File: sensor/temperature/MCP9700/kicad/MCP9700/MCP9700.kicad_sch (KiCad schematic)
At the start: 13 parts, among them U1 MCP9700x-ETT, U3 PIC16F1455

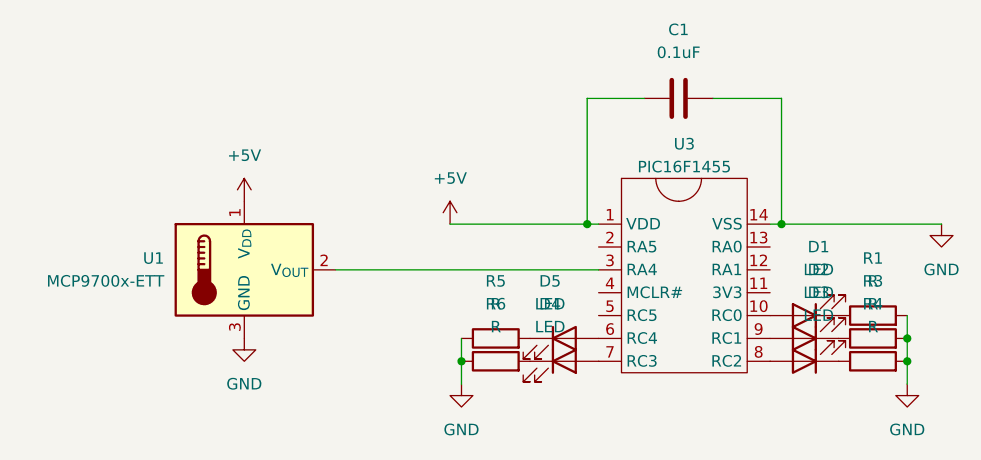
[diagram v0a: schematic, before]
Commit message: update
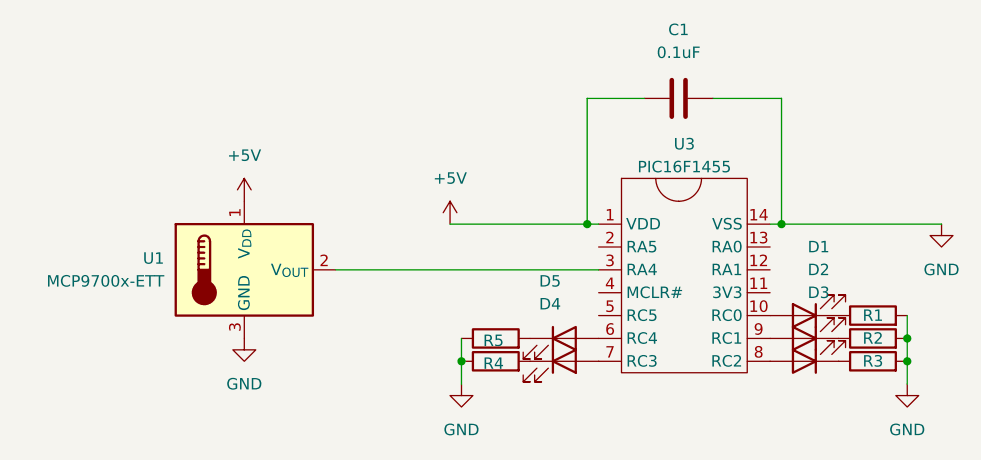
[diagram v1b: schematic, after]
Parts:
- renumbered R3 to R2, R4 to R3, R6 to R4
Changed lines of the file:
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@@
 					(size 1.27 1.27)
 				)
+				(hide yes)
 			)
 		)
@@
 					(size 1.27 1.27)
 				)
+				(hide yes)
 			)
 		)
@@
 		(on_board yes)
 		(dnp no)
-		(fields_autoplaced yes)
 		(property "Reference" "R1"
-			(at 114.3 44.45 90)
+			(at 114.3 50.8 90)
 			(effects
 				(font
@@
 					(size 1.27 1.27)
 				)
+				(hide yes)
 			)
 		)
@@
 		(on_board yes)
 		(dnp no)
-		(fields_autoplaced yes)
-		(property "Reference" "R4"
-			(at 114.3 49.53 90)
+		(property "Reference" "R3"
+			(at 114.3 55.88 90)
 			(effects
 				(font
@@
 					(size 1.27 1.27)
 				)
+				(hide yes)
 			)
 		)
@@
 			(project "MCP9700"
 				(path "/404faf25-665b-4e5e-b4dc-0f02329db52a"
-					(reference "R4")
+					(reference "R3")
 					(unit 1)
 				)
@@
 					(size 1.27 1.27)
 				)
+				(hide yes)
 			)
 		)
@@
 					(size 1.27 1.27)
 				)
+				(hide yes)
 			)
 		)
@@
 		(on_board yes)
 		(dnp no)
-		(fields_autoplaced yes)
-		(property "Reference" "R3"
-			(at 114.3 46.99 90)
+		(property "Reference" "R2"
+			(at 114.3 53.34 90)
 			(effects
 				(font
@@
 					(size 1.27 1.27)
 				)
+				(hide yes)
 			)
 		)
@@
 			(project "MCP9700"
 				(path "/404faf25-665b-4e5e-b4dc-0f02329db52a"
-					(reference "R3")
+					(reference "R2")
 					(unit 1)
 				)
@@
 		(on_board yes)
 		(dnp no)
-		(fields_autoplaced yes)
-		(property "Reference" "R6"
-			(at 72.39 49.53 90)
+		(property "Reference" "R4"
+			(at 72.136 56.134 90)
 			(effects
 				(font
@@
 					(size 1.27 1.27)
 				)
+				(hide yes)
 			)
 		)
@@
 			(project "MCP9700"
 				(path "/404faf25-665b-4e5e-b4dc-0f02329db52a"
-					(reference "R6")
+					(reference "R4")
 					(unit 1)
 				)
@@
 					(size 1.27 1.27)
 				)
+				(hide yes)
 			)
 		)
@@
 		(on_board yes)
 		(dnp no)
-		(fields_autoplaced yes)
 		(property "Reference" "R5"
-			(at 72.39 46.99 90)
+			(at 72.136 53.594 90)
 			(effects
 				(font
@@
 					(size 1.27 1.27)
 				)
-			)
-		)
+				(hide yes)
+			)
+		)
